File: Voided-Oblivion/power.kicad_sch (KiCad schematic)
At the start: 133 parts, among them Q1 AO3401, Q10 BC847B, Q11 BC847B, Q13 NCE4009S, Q14 NCE4009S, Q2 AO4407A, Q3 BC857, Q4 AO4407A, Q5 AO4407A, Q6 AO4407A, Q7 AO4407A, Q8 BC847B, Q9 BC847B, U10 TLV431BQDBZR, U11 LM2903, U12 AP2171WG-7, U13 TPD2E2U06DRL, U14 TPD2E2U06DRL, U15 LM66100DCKT, U16 AP2171WG-7, U17 LM74700QDDF, U18 LM74700QDDF, U2 TS3USB30ERSWR, U5 TPS54302, U6 TPS54302, U7 TLV76733DRVR, U9 LM66100DCKT

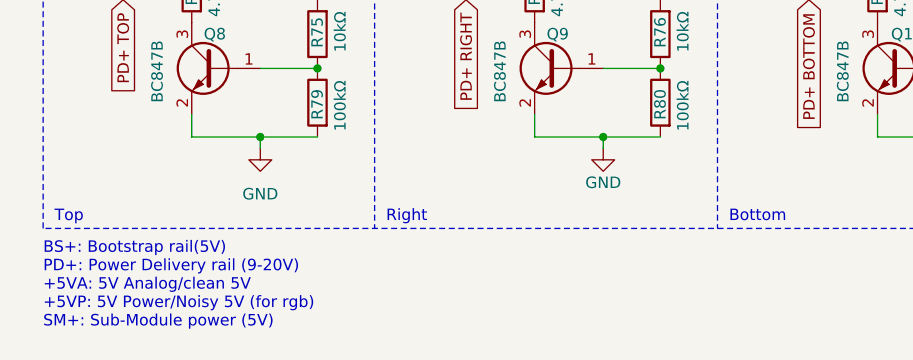
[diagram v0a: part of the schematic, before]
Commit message: pcb almooost done
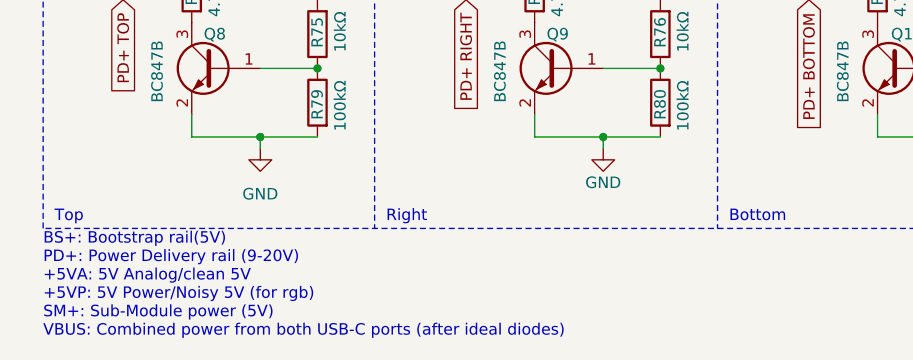
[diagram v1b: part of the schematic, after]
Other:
- note added: "BS+: Bootstrap rail(5V) PD+: Power Delivery rail (9-20V) +5VA: 5V Analog/clean 5V +5VP: 5V Power/Noisy 5V (for rgb) SM+: Sub-Module power (5V) VBUS: Combined power from both USB-C ports (after ideal diodes)"
- note removed: "BS+: Bootstrap rail(5V) PD+: Power Delivery rail (9-20V) +5VA: 5V Analog/clean 5V +5VP: 5V Power/Noisy 5V (for rgb) SM+: Sub-Module power (5V)"
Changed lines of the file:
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@@
 		)
 	)
-	(text "BS+: Bootstrap rail(5V)\nPD+: Power Delivery rail (9-20V)\n+5VA: 5V Analog/clean 5V\n+5VP: 5V Power/Noisy 5V (for rgb)\nSM+: Sub-Module power (5V)"
+	(text "BS+: Bootstrap rail(5V)\nPD+: Power Delivery rail (9-20V)\n+5VA: 5V Analog/clean 5V\n+5VP: 5V Power/Noisy 5V (for rgb)\nSM+: Sub-Module power (5V)\nVBUS: Combined power from both USB-C ports (after ideal diodes)"
 		(exclude_from_sim no)
 		(at 16.51 274.32 0)
